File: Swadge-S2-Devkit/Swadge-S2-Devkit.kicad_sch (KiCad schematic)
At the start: 99 parts, among them J1 SAO, J3 Conn_01x05_Male, P1 USB_C_Plug_USB2.0, Q1 Q_PMOS_GSD, SW1 TS-1109S-A-A, SW2 TS-1109S-A-A, SW3 TS-1109S-A-A, SW4 TS-1109S-A-A, SW5 TS-1109S-A-A, SW6 TS-1109S-A-A, SW7 B3FS-4002P, SW8 B3FS-4002P, SW9 SW_SPDT_1825232-1, U1 ESP32-S2-SOLO, U2 RB017A1505A, U3 MT3410, U4 RB0154A1201A, U5 RB017A1505A_Connector, U6 Controller_Shields, U7 GENERIC_LDO_2.8, U8 QMA7981

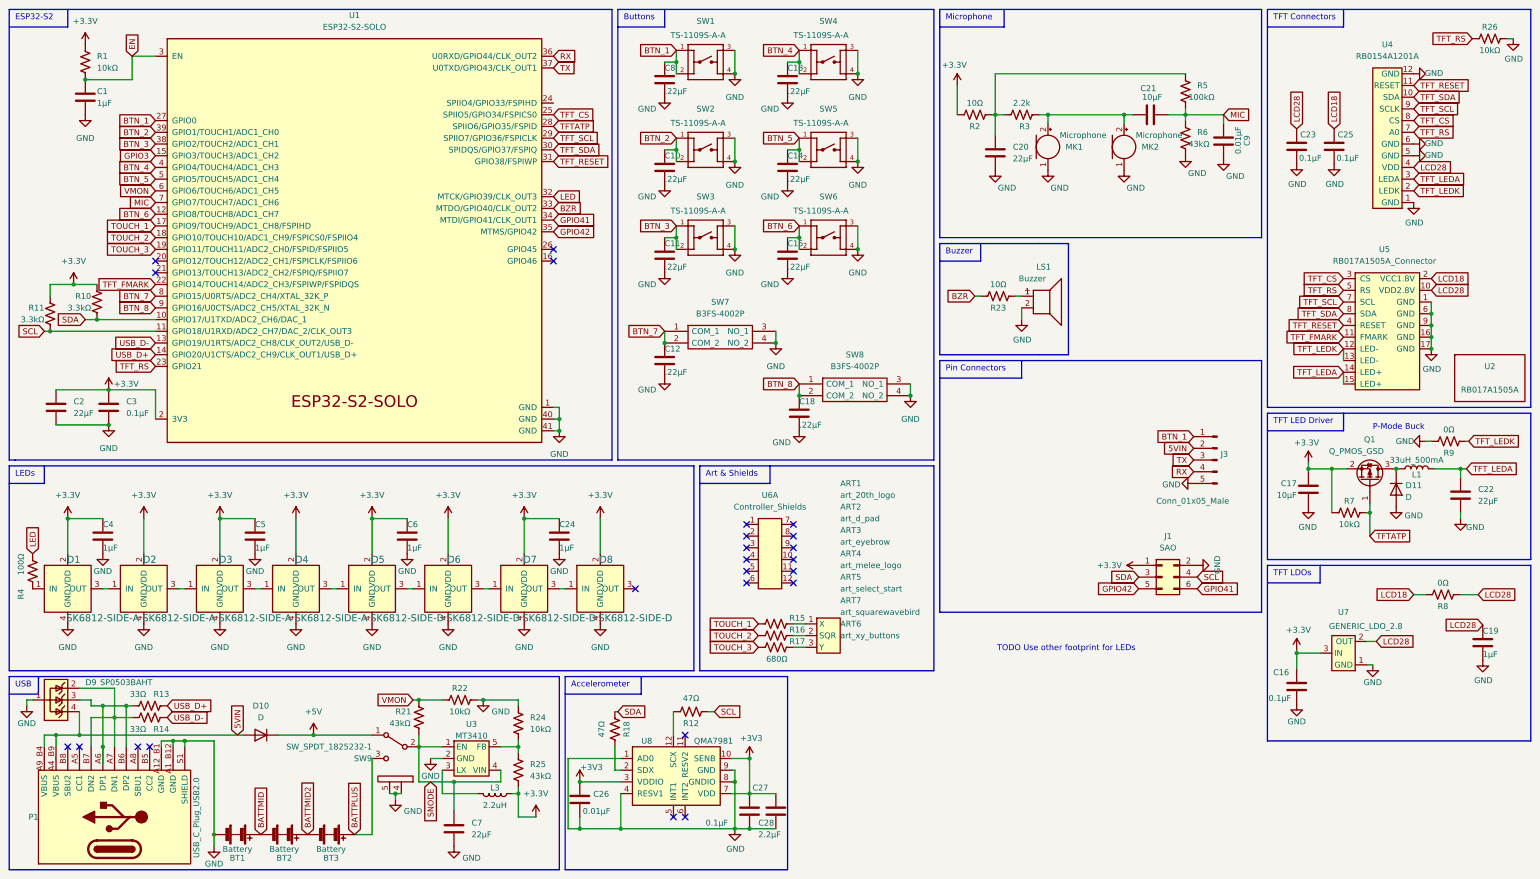
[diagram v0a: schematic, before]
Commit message: Bump swadge.
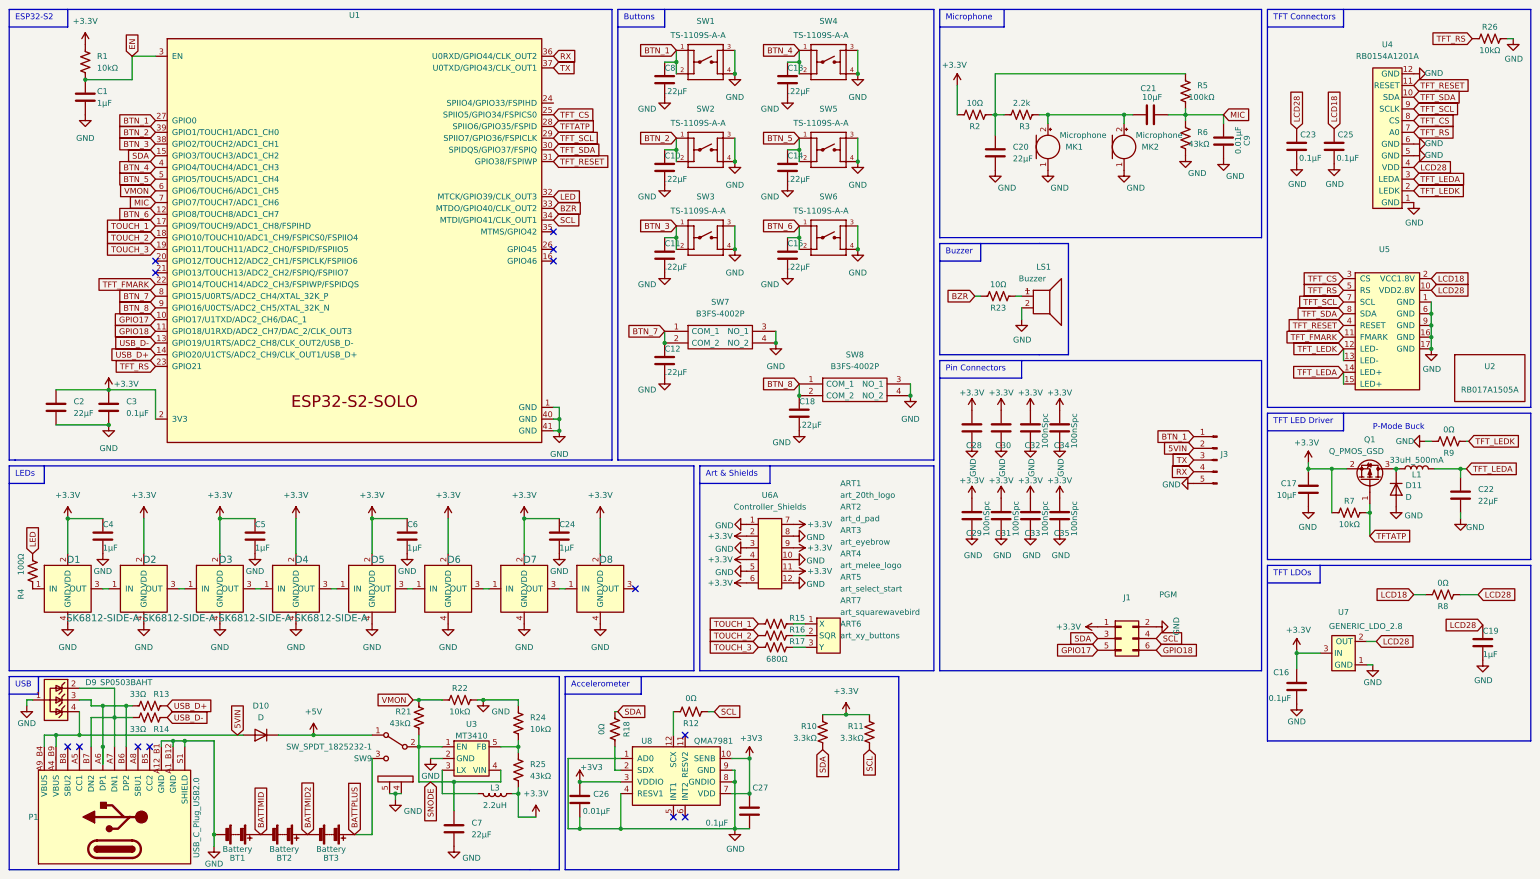
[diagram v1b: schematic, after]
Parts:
- removed C28: 2.2μF, Swadge_Parts:C_0603_1608Metric, symbol Swadge_Parts:C
- added C28, C30: (no value), symbol Device:C
- added C29, C31, C32, C33, C34, C35: 100nSpc, Capacitor_SMD:C_1210_3225Metric_Pad1.33x2.70mm_HandSolder, symbol Device:C
- D5, D6, D7, D8: value SK6812-SIDE-D -> (none); footprint Swadge_Parts:SK6812D_SIDE -> (none); LCSC C2890037 -> C2890041
- J1: value SAO -> (none); footprint Swadge_Parts:PinHeader_2x03_P2.54mm_Vertical -> (none)
- J3: value Conn_01x05_Male -> PGM
- R12, R18: value 47Ω -> 0Ω; LCSC C254549 -> C21189
- U1: value ESP32-S2-SOLO -> (none); footprint Swadge_Parts:ESP32-S2-SOLO -> (none); LCSC (none) -> C3013947
- U5: value RB017A1505A_Connector -> (none); footprint Swadge_Parts:HCTL HC-FPC-03-10-15RLTAG -> (none); LCSC C3012328 -> C3029632
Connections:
- net GPIO3 is gone; now on net SDA: U1.15 (GPIO3/TOUCH3/ADC1_CH2)
- net +3V3: now also R10.2, R11.1, U6.11, U6.2, U6.4, U6.6, U6.7, U6.9, C28.1, C29.1, C30.1, C31.1, C32.1, C33.1, C34.1, C35.1; no longer R10.1, R11.2
- net GND: now also U6.1, U6.10, U6.12, U6.3, U6.5, U6.8, C28.2, C29.2, C30.2, C31.2, C32.2, C33.2, C34.2, C35.2
- net SCL: now also R11.2, U1.34 (MTDI/GPIO41/CLK_OUT1); no longer R11.1, U1.11 (GPIO18/U1RXD/ADC2_CH7/DAC_2/CLK_OUT3)
- net SDA: now also R10.1; no longer R10.2, U1.10 (GPIO17/U1TXD/ADC2_CH6/DAC_1)
- net GPIO41 renamed GPIO18
- net GPIO18: now also U1.11 (GPIO18/U1RXD/ADC2_CH7/DAC_2/CLK_OUT3); no longer U1.34 (MTDI/GPIO41/CLK_OUT1)
- net GPIO42: no longer names the net of U1.35 (MTMS/GPIO42)
- net GPIO42: no longer J1.5 (Pin_5)
- new net GPIO17: J1.5 (Pin_5), U1.10 (GPIO17/U1TXD/ADC2_CH6/DAC_1)
- no-connect marks 24 -> 13
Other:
- note removed: "TODO Use other footprint for LEDs"
- moved on the sheet: J1
